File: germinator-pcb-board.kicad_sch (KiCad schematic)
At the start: 10 parts, among them J1 Conn_01x15_Socket, J2 Conn_01x15_Socket, J3 Screw_Terminal_01x04, J4 Screw_Terminal_01x03, J5 Screw_Terminal_01x03, J6 Screw_Terminal_01x03, J7 Screw_Terminal_01x03, U1 ESP32-DEVKIT-V1

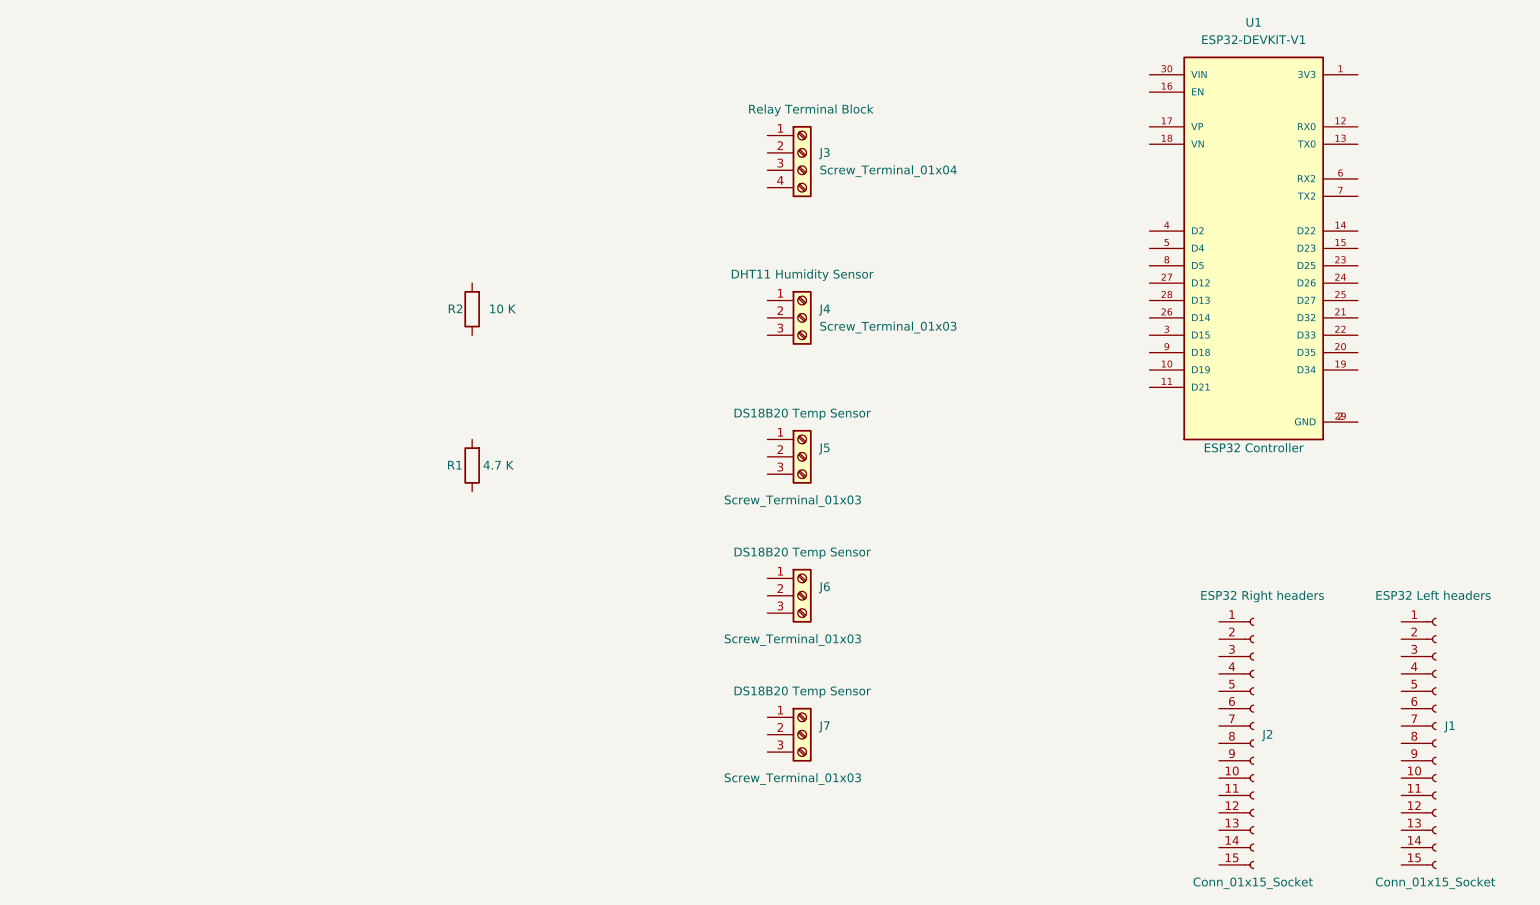
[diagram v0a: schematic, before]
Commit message: Schematics step 4: Wiring
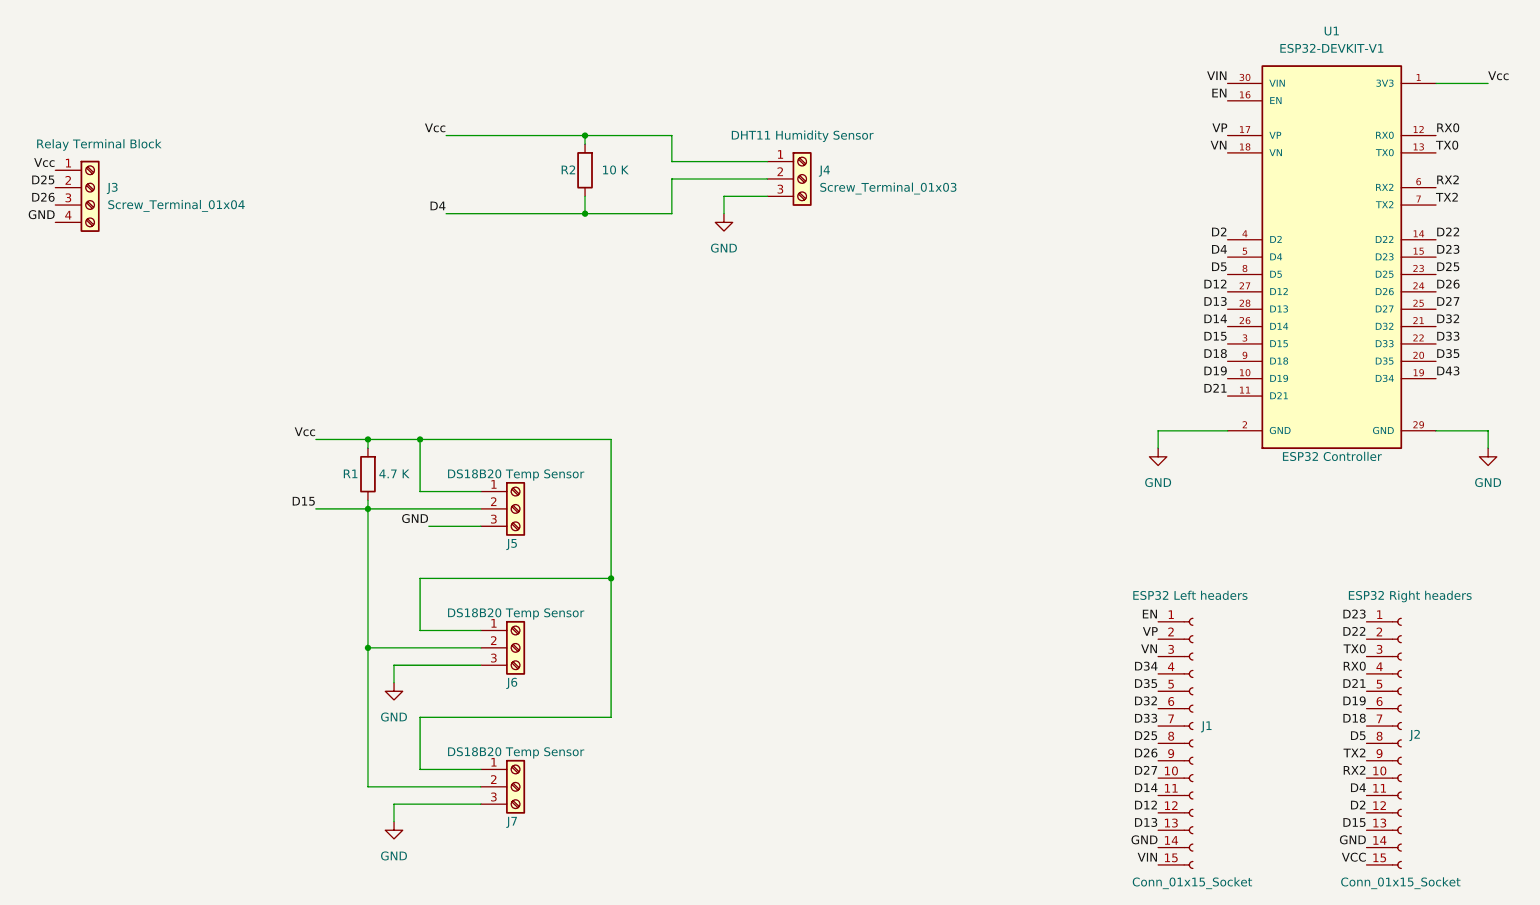
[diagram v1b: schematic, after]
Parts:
- U1: footprint germinator-pcb-board-libraries:ESP32_DEVKIT_V1 -> ESP32-DEVKIT-V1:MODULE_ESP32_DEVKIT_V1; Availability (none) -> Not in stock; Check_prices (none) -> https://www.snapeda.com/parts/ESP32-DEVKIT-V1/Do+it/view-pa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; Description_1 (none) -> Dual core, Wi-Fi: 2.4 GHz up to 150 Mbits/s,BLE (Bluetooth 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; MAXIMUM_PACKAGE_HEIGHT (none) -> 6.8 mm; MF (none) -> Do it; MP (none) -> ESP32-DEVKIT-V1; PARTREV (none) -> N/A; Package (none) -> None; Price (none) -> None; STANDARD (none) -> Manufacturer Recommendations; SnapEDA_Link (none) -> https://www.snapeda.com/parts/ESP32-DEVKIT-V1/Do+it/view-pa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
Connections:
- net Vcc: now reaches J6.1 (Pin_1)
- net Vcc: now also J3.1 (Pin_1), J4.1 (Pin_1), J5.1 (Pin_1), J7.1 (Pin_1), R1.2, R2.2, U1.1 (3V3)
- net D15: now reaches J6.2 (Pin_2)
- net D15: now also J2.13 (Pin_13), J5.2 (Pin_2), J7.2 (Pin_2), R1.1, U1.3 (D15)
- net GND: now reaches J6.3 (Pin_3)
- net GND: now also J1.14 (Pin_14), J2.14 (Pin_14), J3.4 (Pin_4), J4.3 (Pin_3), J5.3 (Pin_3), J7.3 (Pin_3), U1.2 (GND), U1.29 (GND)
- net D25: now reaches J3.2 (Pin_2)
- net D25: now also J1.8 (Pin_8), U1.23 (D25)
- net D26: now reaches J3.3 (Pin_3)
- net D26: now also J1.9 (Pin_9), U1.24 (D26)
- net EN: now reaches J1.1 (Pin_1)
- net EN: now also U1.16 (EN)
- net D27: now reaches J1.10 (Pin_10)
- net D27: now also U1.25 (D27)
- net D14: now reaches J1.11 (Pin_11)
- net D14: now also U1.26 (D14)
- net D12: now reaches J1.12 (Pin_12)
- net D12: now also U1.27 (D12)
- net D13: now reaches J1.13 (Pin_13)
- net D13: now also U1.28 (D13)
- net VIN: now reaches J1.15 (Pin_15)
- net VIN: now also U1.30 (VIN)
- net VP: now reaches J1.2 (Pin_2)
- net VP: now also U1.17 (VP)
- net VN: now reaches J1.3 (Pin_3)
- net VN: now also U1.18 (VN)
- net D34: now reaches J1.4 (Pin_4)
- net D35: now reaches J1.5 (Pin_5)
- net D35: now also U1.20 (D35)
- net D32: now reaches J1.6 (Pin_6)
- net D32: now also U1.21 (D32)
- net D33: now reaches J1.7 (Pin_7)
- net D33: now also U1.22 (D33)
- net D23: now reaches J2.1 (Pin_1)
- net D23: now also U1.15 (D23)
- net RX2: now reaches J2.10 (Pin_10)
- net RX2: now also U1.6 (RX2)
- net D4: now reaches J2.11 (Pin_11)
- net D4: now also J4.2 (Pin_2), R2.1, U1.5 (D4)
- net D2: now reaches J2.12 (Pin_12)
- net D2: now also U1.4 (D2)
- net VCC: now reaches J2.15 (Pin_15)
- net D22: now reaches J2.2 (Pin_2)
- net D22: now also U1.14 (D22)
- net TX0: now reaches J2.3 (Pin_3)
- net TX0: now also U1.13 (TX0)
- net RX0: now reaches J2.4 (Pin_4)
- net RX0: now also U1.12 (RX0)
- net D21: now reaches J2.5 (Pin_5)
- net D21: now also U1.11 (D21)
- net D19: now reaches J2.6 (Pin_6)
- net D19: now also U1.10 (D19)
- net D18: now reaches J2.7 (Pin_7)
- net D18: now also U1.9 (D18)
- net D5: now reaches J2.8 (Pin_8)
- net D5: now also U1.8 (D5)
- net TX2: now reaches J2.9 (Pin_9)
- net TX2: now also U1.7 (TX2)
- net D43: now reaches U1.19 (D34)
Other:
- moved on the sheet: J1, J2, J3, J4, J5, J6, J7, R1, R2
